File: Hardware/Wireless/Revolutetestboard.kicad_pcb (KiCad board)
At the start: 4 copper layers, 54 x 85.6 mm, 104 parts, among them J1 -, J2 +, J3 USB_C_Receptacle_USB2.0, J4 Conn_01x02_Pin, J5 USB_C_Receptacle_USB2.0, Q1 NMOS, Q2 NMOS-CSD17381F4, Q3 NMOS-CSD17381F4, Q4 PMOS-CSD25483F4, Q5 PMOS-CSD25483F4, SW1 SW_DIP_x05, U10 Button, U11 LSM6DSO, U12 STM32F103C8Tx, U13 AP2112K-3.3, U14 Conn_01x14_Socket, U2 nrf52833_qfn40, U3 AS5600, U4 MIC5504, U5 BQ24075RGT, U6 Button, U7 Conn_01x14_Socket, U8 Button, U9 Button, X1 32.768 kHz, X2 32MHZ, Y1 32.768KHZ, Y2 8Mhz

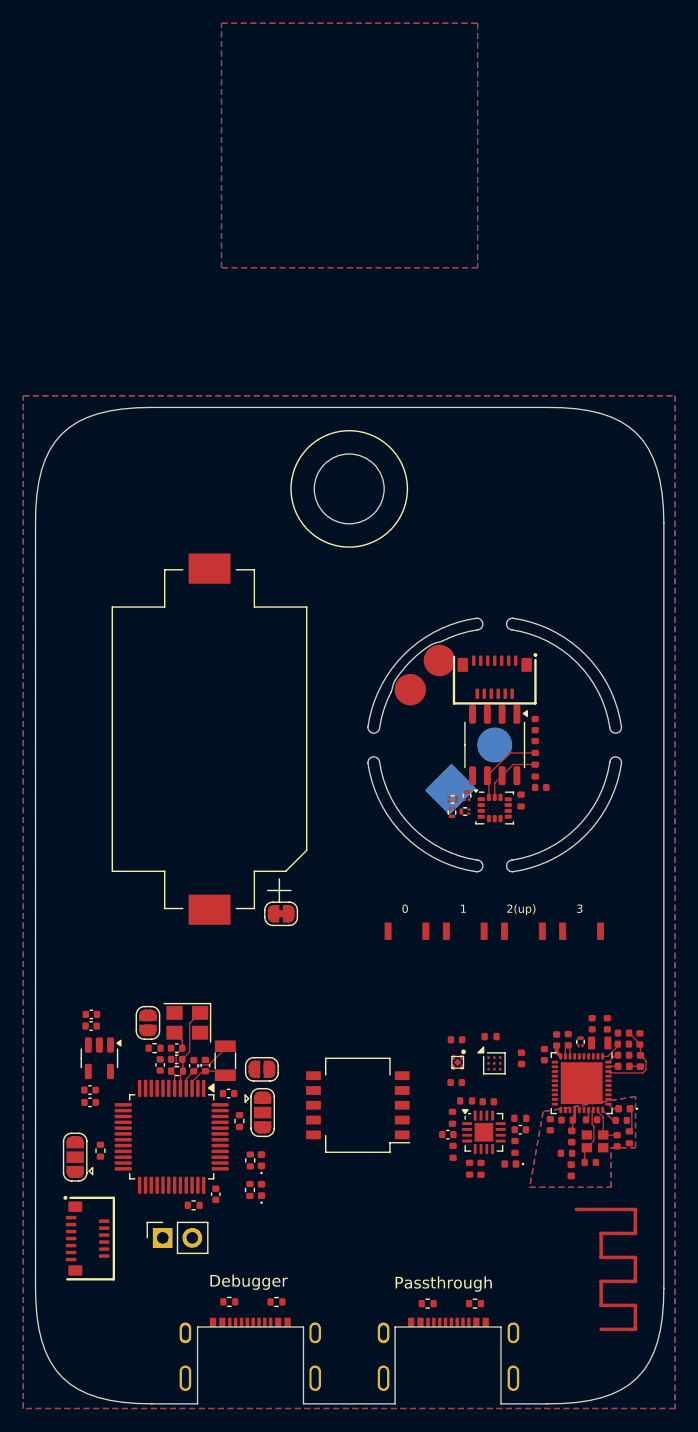
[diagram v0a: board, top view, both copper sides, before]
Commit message: new flex and new pcbs
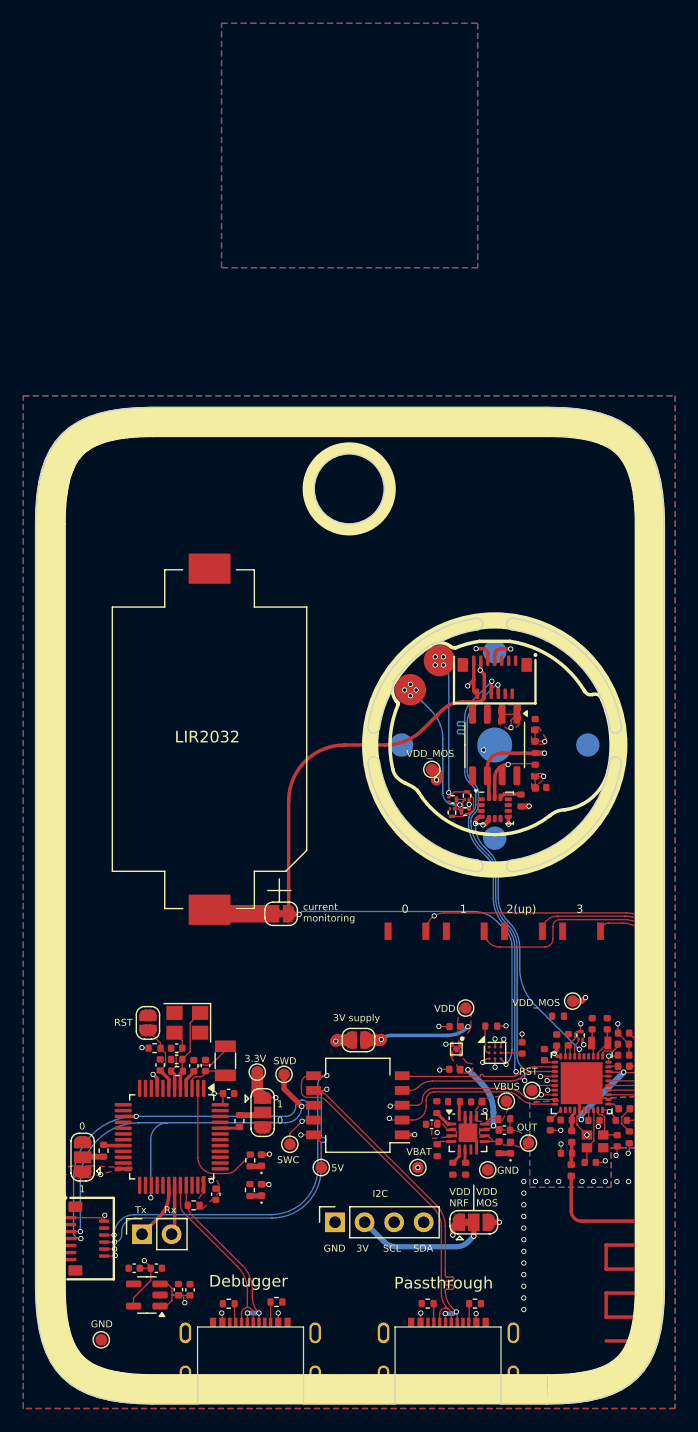
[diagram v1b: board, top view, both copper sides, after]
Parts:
- removed ? (x2): , 
- added J6: Conn_01x04_Socket, Connector_PinSocket_2.54mm:PinSocket_1x04_P2.54mm_Vertical, F.Cu at (134.8, 140.0)
- added JP6: Jumper_3_Bridged12, Jumper:SolderJumper-3_P1.3mm_Bridged12_RoundedPad1.0x1.5mm, F.Cu at (146.7, 140.0)
- added R23: 2M, Library:Resistor_0402_1005M-nosilk, F.Cu at (153.9, 122.3)
- added SW2: SW_Push, Library:16mmCompButton, B.Cu at (148.5, 99.0)
- added TP1: TestPoint, TestPoint:TestPoint_Pad_D1.0mm, F.Cu at (151.7, 128.7)
- added TP10: TestPoint, TestPoint:TestPoint_Pad_D1.0mm, F.Cu at (146.0, 121.6)
- added TP11: TestPoint, TestPoint:TestPoint_Pad_D1.0mm, F.Cu at (155.2, 121.0)
- added TP12: TestPoint, TestPoint:TestPoint_Pad_D1.0mm, F.Cu at (149.5, 129.6)
- added TP13: TestPoint, TestPoint:TestPoint_Pad_D1.0mm, F.Cu at (141.9, 135.3)
- added TP2: TestPoint, TestPoint:TestPoint_Pad_D1.0mm, F.Cu at (147.9, 135.5)
- added TP3: TestPoint, TestPoint:TestPoint_Pad_D1.0mm, F.Cu at (133.6, 135.3)
- added TP4: TestPoint, TestPoint:TestPoint_Pad_D1.0mm, F.Cu at (114.7, 150.1)
- added TP5: TestPoint, TestPoint:TestPoint_Pad_D1.0mm, F.Cu at (128.1, 127.1)
- added TP6: TestPoint, TestPoint:TestPoint_Pad_D1.0mm, F.Cu at (130.9, 133.3)
- added TP7: TestPoint, TestPoint:TestPoint_Pad_D1.0mm, F.Cu at (130.4, 127.3)
- added TP8: TestPoint, TestPoint:TestPoint_Pad_D1.0mm, F.Cu at (151.4, 133.2)
- added TP9: TestPoint, TestPoint:TestPoint_Pad_D1.0mm, F.Cu at (143.1, 101.1)
- Q1: value NMOS -> PMOS-CSD25483F4
- moved C28 25.1 mm to (122.3, 145.8), turned to -90 degrees
- moved C29 23.9 mm to (121.3, 145.8), turned to -90 degrees
- moved U13 20.7 mm to (118.6, 146.3), turned to 180 degrees
- moved C32 15.8 mm to (117.5, 143.9)
- moved C33 15.3 mm to (119.4, 143.9), turned to 180 degrees
- moved JP4 8.67 mm to (136.8, 124.3), turned to 0 degrees
- moved J4 1.81 mm to (118.2, 141.0)
- moved C25 1.65 mm to (143.1, 131.6)
- moved TH1 1.62 mm to (143.5, 130.1)
- moved R7 1.44 mm to (144.9, 135.4)
- moved D2 1.41 mm to (149.9, 133.6), turned to 90 degrees
- moved R3 1.37 mm to (143.6, 133.8)
- moved R4 1.37 mm to (149.3, 131.1)
- moved R9 1.37 mm to (148.9, 133.6)
- moved U5 1.37 mm to (146.2, 132.3)
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- renumbered AE** to Antenna
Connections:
- Q1 pad 2: MOS_VDD -> VDD_nRF
- Q1 pad 3: VDD_nRF -> MOS_VDD
- SW1 pad 1: unconnected-(SW1-Pad1) -> VBUS
- SW1 pad 2: unconnected-(SW1-Pad2) -> swc
- SW1 pad 3: unconnected-(SW1-Pad3) -> swd
- SW1 pad 4: unconnected-(SW1-Pad4) -> D+
- SW1 pad 5: unconnected-(SW1-Pad5) -> D-
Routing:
- net swc: track 0.00 -> 67.4 mm, vias 0 -> 2
- net swd: track 0.00 -> 65.9 mm, vias 0 -> 2
- net Batteryin: track 0.00 -> 65.4 mm, vias 0 -> 3
- net MOS_VDD: track 0.00 -> 61.2 mm, vias 0 -> 10
- net VBUS: track 1.06 -> 61.9 mm, vias 0 -> 5
- net /USBDM2: track 0.00 -> 60.5 mm, vias 0 -> 2
- net /USBDP2: track 0.00 -> 60.2 mm, vias 0 -> 4
- net P0.28: track 0.00 -> 57.8 mm, vias 0 -> 2
- net P0.15: track 5.37 -> 59.0 mm, vias 0 -> 3
- net D-: track 0.00 -> 53.2 mm, vias 0 -> 2
- net P0.17: track 6.84 -> 59.8 mm, vias 0 -> 3
- net D+: track 0.00 -> 52.0 mm, vias 0 -> 2
- net /B14: track 0.00 -> 40.4 mm, vias 0 -> 3
- net /A5: track 0.00 -> 36.5 mm, vias 0 -> 3
- net P0.30: track 0.00 -> 33.6 mm
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- added copper zone on F.Cu, net 3.3V
- added copper zone on In2.Cu, net 3.3V
- added copper zone on In2.Cu, net 5V
- added copper zone on F.Cu, net MOS_VDD
- added copper zone on In2.Cu, net MOS_VDD
- added copper zone on F.Cu, net OUT
- added copper zone on F.Cu, net VBUS
- added copper zone on F.Cu, net VDD_nRF
- added copper zone on In2.Cu, net VDD_nRF
- added copper zone on F.Cu, net vBAT
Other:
- board text added: "3.3V"
- board text added: "3V"
- board text added: "3V supply"
- board text added: "5V"
- board text added: "FOR BOOTLOADER, Boot0=1 Boot1=0"
- board text added: "FOR OPERATION, Boot0=0 Boot1=0"
- board text added: "GND"
- board text added: "I2C"
- board text added: "LIR2032"
- board text added: "OUT"
- board text added: "Oct 20 2024"
- board text added: "RST"
- board text added: "Rev1"
- board text added: "Rx"
- board text added: "SCL"
- board text added: "SDA"
- board text added: "SWC"
- board text added: "SWD"
- board text added: "Test"
- board text added: "Tongtong.inc"
- board text added: "Tx"
- board text added: "VBAT"
- board text added: "VBUS"
- board text added: "VDD"
- board text added: "VDD MOS"
- board text added: "VDD NRF"
- board text added: "VDD_MOS"
- board text added: "current monitoring"
